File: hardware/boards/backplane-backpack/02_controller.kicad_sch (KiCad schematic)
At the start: 12 parts, among them J10 SWD (TBD), U1 STM32C092FCP6

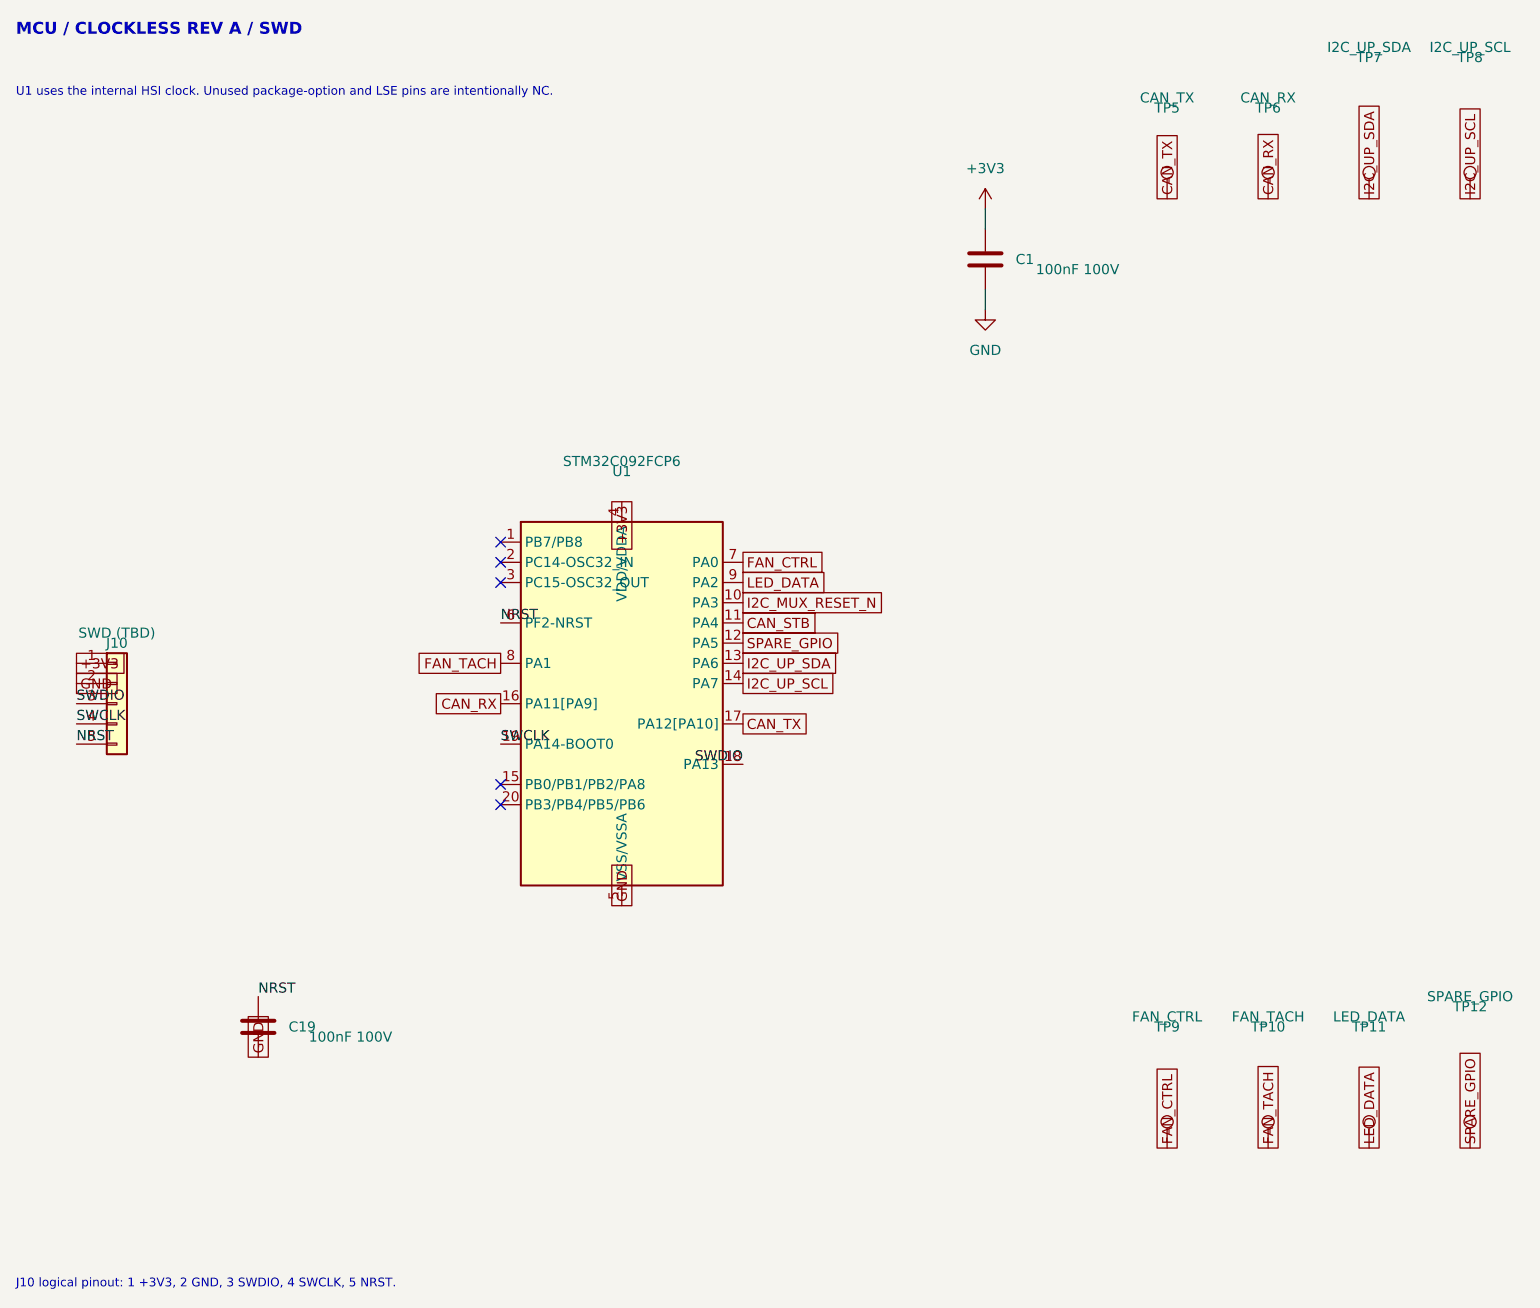
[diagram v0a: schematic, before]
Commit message: chore: checkpoint workspace changes
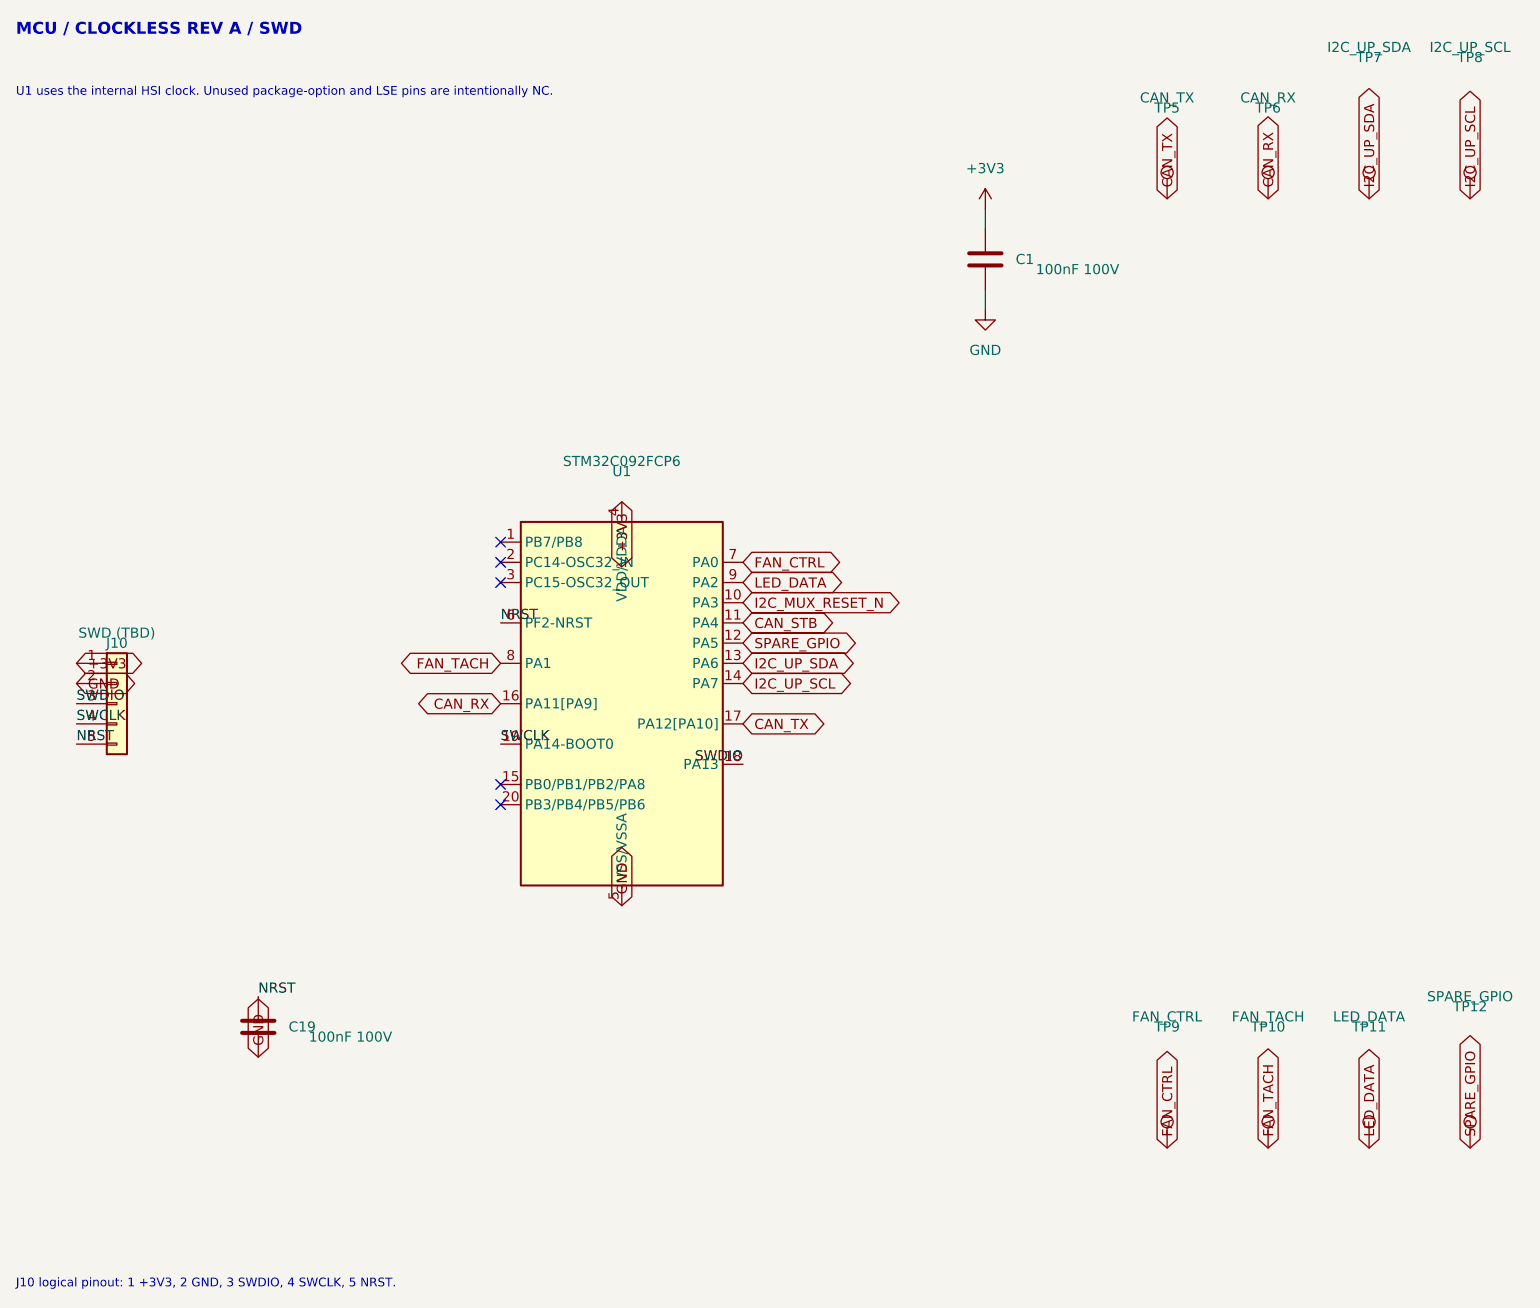
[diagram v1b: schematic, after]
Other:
- company: (none) -> Karl Quinsland
- title: MCU and Debug -> Backplane Backpack
